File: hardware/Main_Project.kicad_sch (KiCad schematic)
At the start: 79 parts, among them J1 Motors_R, J10 BBBBBBBONUSROUND, J11 Power_Distro, J12 Power_Distro, J13 Power_Distro, J14 Power_Distro, J15 Color_Sensor, J16 Color_Sensor, J17 Magnet, J18 FRDM input, J19 Magnet_Power, J2 Motors_L, J3 Power_Outputs, J4 Motor_Control, J5 Motor_Power, J6 Motor_Power, J7 Motor_Control, J8 Color_Sensor, J9 Magnet?, Q2 BC547, Q3 IRF540N, U1 L7805, U2 L298N

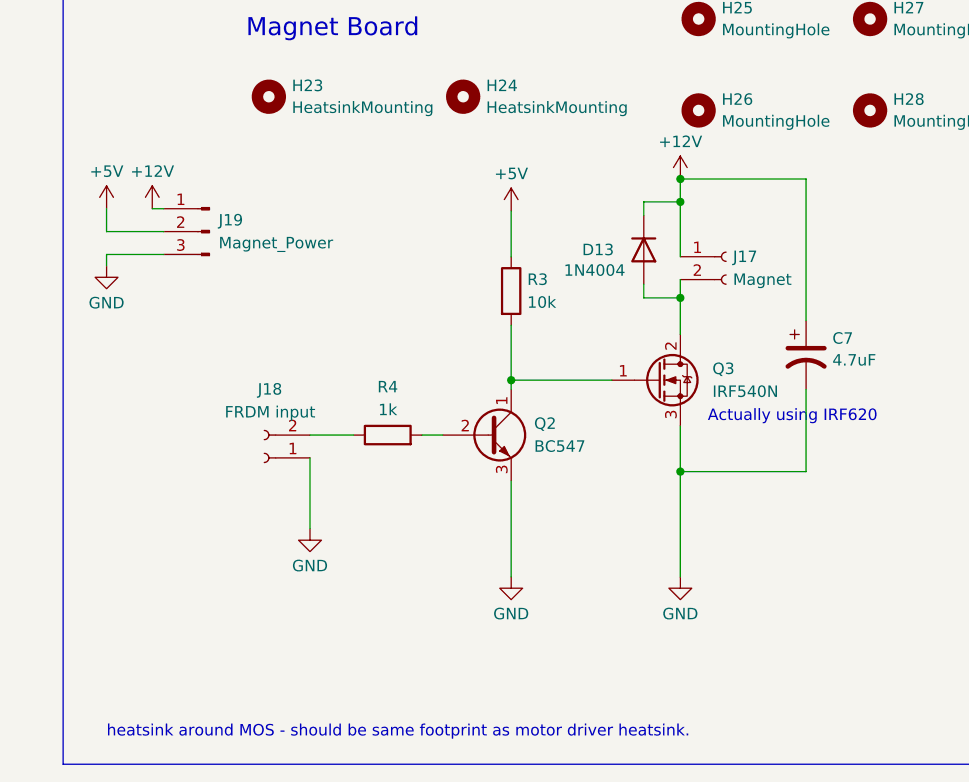
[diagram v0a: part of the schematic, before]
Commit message: Magnet board
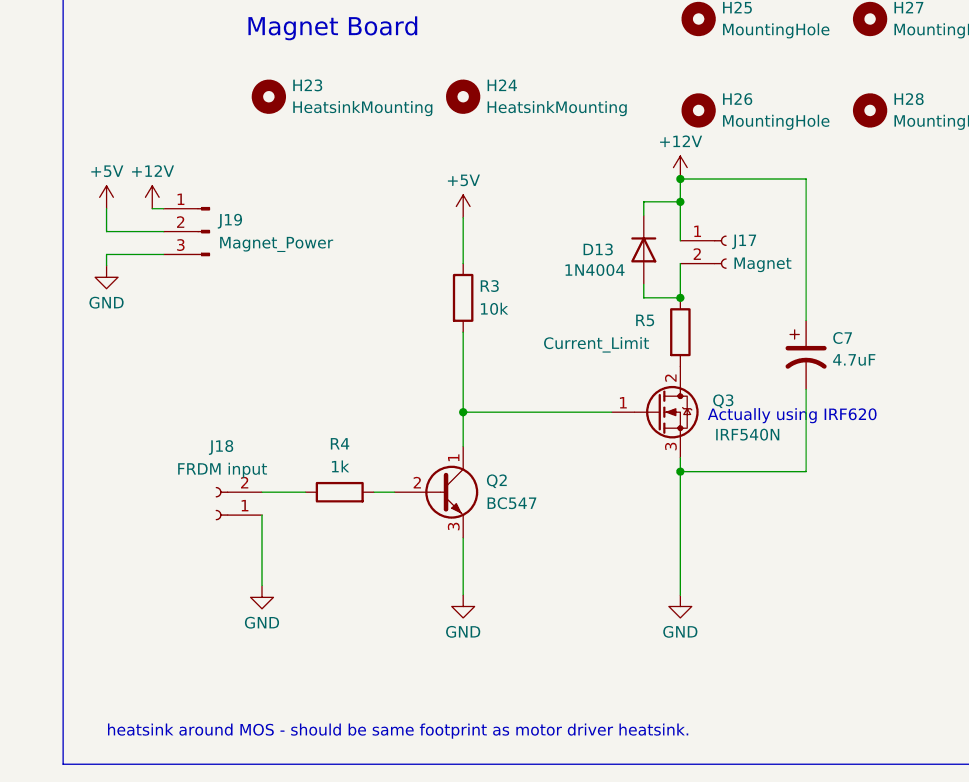
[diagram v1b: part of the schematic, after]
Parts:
- added R5: Current_Limit, Resistor_THT:R_Axial_DIN0207_L6.3mm_D2.5mm_P10.16mm_Horizontal, symbol Device:R
- J18: footprint TerminalBlock:TerminalBlock_bornier-2_P5.08mm -> Connector_Molex:Molex_KK-254_AE-6410-02A_1x02_P2.54mm_Vertical
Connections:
- net at D13.2 (A), J17.2 (Pin_2): now also R5.1; no longer Q3.2 (D)
- new net: Q3.2 (D), R5.2
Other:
- moved on the sheet: J17, J18, Q2, Q3, R3, R4

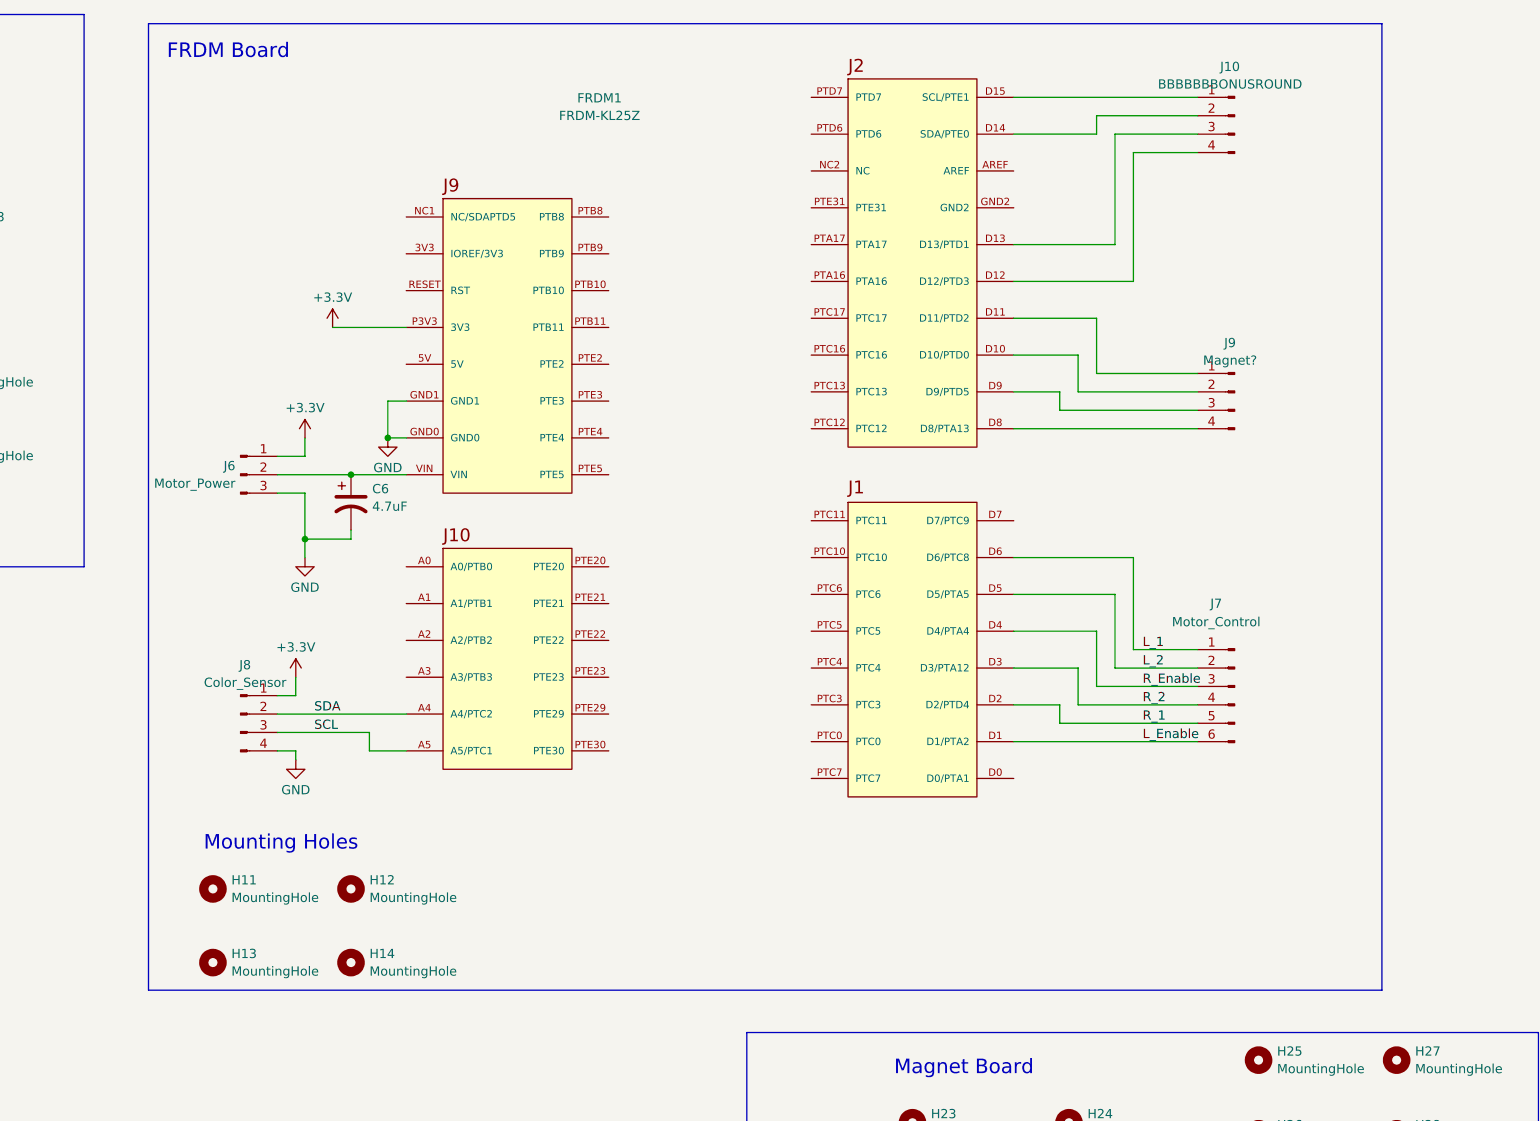
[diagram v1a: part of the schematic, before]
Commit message: New FRDM Board
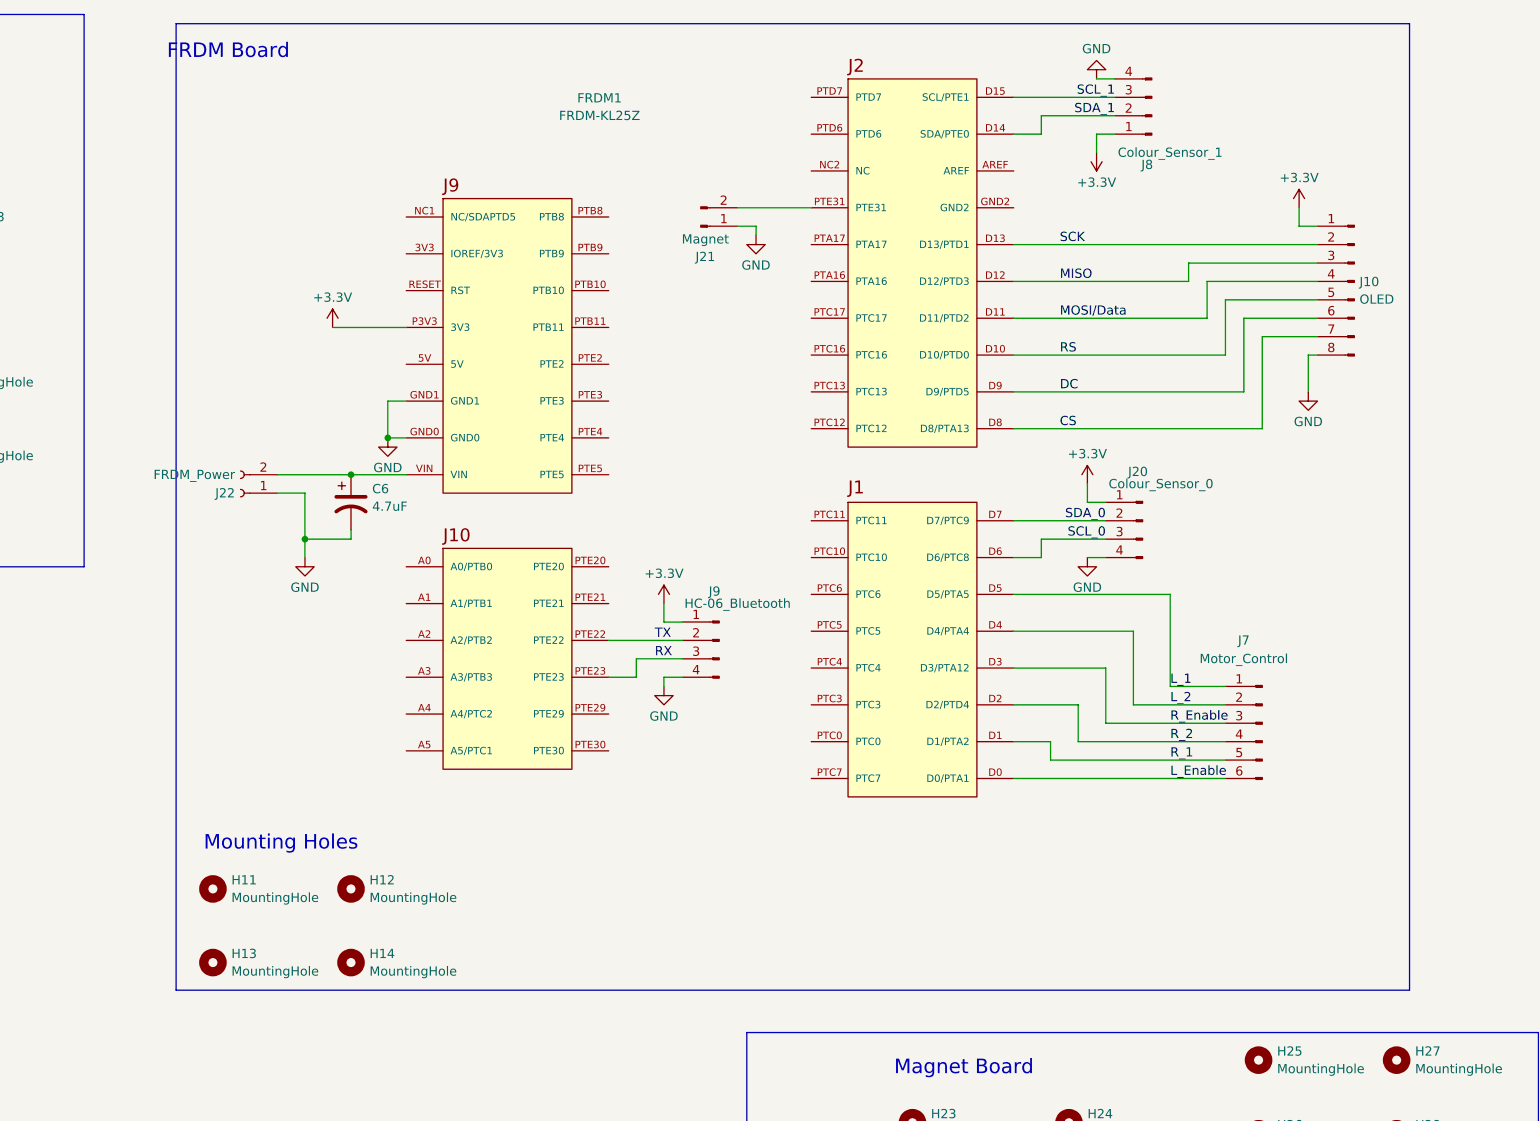
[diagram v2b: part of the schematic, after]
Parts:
- removed J10: BBBBBBBONUSROUND, Connector_Molex:Molex_KK-254_AE-6410-04A_1x04_P2.54mm_Vertical, symbol Connector:Conn_01x04_Pin
- removed J6: Motor_Power, TerminalBlock:TerminalBlock_bornier-3_P5.08mm, symbol Connector:Conn_01x03_Pin
- added J10: OLED, Connector_Molex:Molex_KK-254_AE-6410-08A_1x08_P2.54mm_Vertical, symbol Connector:Conn_01x08_Pin
- added J20: Colour_Sensor_0, Connector_Molex:Molex_KK-254_AE-6410-04A_1x04_P2.54mm_Vertical, symbol Connector:Conn_01x04_Pin
- added J21: Magnet, Connector_Molex:Molex_KK-254_AE-6410-02A_1x02_P2.54mm_Vertical, symbol Connector:Conn_01x02_Pin
- added J22: FRDM_Power, TerminalBlock:TerminalBlock_bornier-2_P5.08mm, symbol Connector:Conn_01x02_Socket
- J8: value Color_Sensor -> Colour_Sensor_1
- J9: value Magnet? -> HC-06_Bluetooth
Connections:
- net +3V3: now also J9.1 (Pin_1), J10.1 (Pin_1), J20.1 (Pin_1)
- net GND: now also J9.4 (Pin_4), J10.8 (Pin_8), J20.4 (Pin_4), J21.1 (Pin_1), J22.1 (Pin_1)
- net L_1: now also FRDM1.D5 (D5/PTA5); no longer FRDM1.D6 (D6/PTC8)
- net L_2: now also FRDM1.D4 (D4/PTA4); no longer FRDM1.D5 (D5/PTA5)
- net L_Enable: now also FRDM1.D0 (D0/PTA1); no longer FRDM1.D1 (D1/PTA2)
- net R_1: now also FRDM1.D1 (D1/PTA2); no longer FRDM1.D2 (D2/PTD4)
- net R_2: now also FRDM1.D2 (D2/PTD4); no longer FRDM1.D3 (D3/PTA12)
- net R_Enable: now also FRDM1.D3 (D3/PTA12); no longer FRDM1.D4 (D4/PTA4)
- net SCL_1: now reaches FRDM1.D15 (SCL/PTE1)
- net SCL_1: now also J8.3 (Pin_3)
- net SDA_1: now reaches FRDM1.D14 (SDA/PTE0)
- net SDA_1: now also J8.2 (Pin_2)
- net SCK: now reaches FRDM1.D13 (D13/PTD1)
- net SCK: now also J10.2 (Pin_2)
- net MISO: now reaches FRDM1.D12 (D12/PTD3)
- net MISO: now also J10.3 (Pin_3)
- net at C6.1, FRDM1.VIN: now also J22.2 (Pin_2)
- net MOSI/Data: now reaches FRDM1.D11 (D11/PTD2)
- net MOSI/Data: now also J10.4 (Pin_4); no longer J9.1 (Pin_1)
- net RS: now reaches FRDM1.D10 (D10/PTD0)
- net RS: now also J10.5 (Pin_5); no longer J9.2 (Pin_2)
- net DC: now reaches FRDM1.D9 (D9/PTD5)
- net DC: now also J10.6 (Pin_6); no longer J9.3 (Pin_3)
- net CS: now reaches FRDM1.D8 (D8/PTA13)
- net CS: now also J10.7 (Pin_7); no longer J9.4 (Pin_4)
- net SDA_0: now reaches FRDM1.D7 (D7/PTC9)
- net SDA_0: now also J20.2 (Pin_2)
- net TX: now reaches FRDM1.PTE22
- net TX: now also J9.2 (Pin_2)
- net RX: now reaches FRDM1.PTE23
- net RX: now also J9.3 (Pin_3)
- net at FRDM1.PTE31: now also J21.2 (Pin_2)
- net SCL: no longer names the net of FRDM1.A5 (A5/PTC1)
- net SCL: no longer J8.3 (Pin_3)
- net SDA: no longer names the net of FRDM1.A4 (A4/PTC2)
- net SDA: no longer J8.2 (Pin_2)
- new net SCL_0: FRDM1.D6 (D6/PTC8), J20.3 (Pin_3)
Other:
- moved on the sheet: J7, J8
